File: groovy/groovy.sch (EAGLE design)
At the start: 51 parts, among them J1 USB_MICRO, J2 2_PIN_JST-XH, J3 BL, J4 PWR, J5 FLASH, P1 MICROSD, U1 MCP73831T, U2 AP7312-1833, U3 VS1053, U4 ATMEGA328PB-AUR, Y1 ABM8G-12.288MHZ-18-D2Y-T, Y2 8MHz

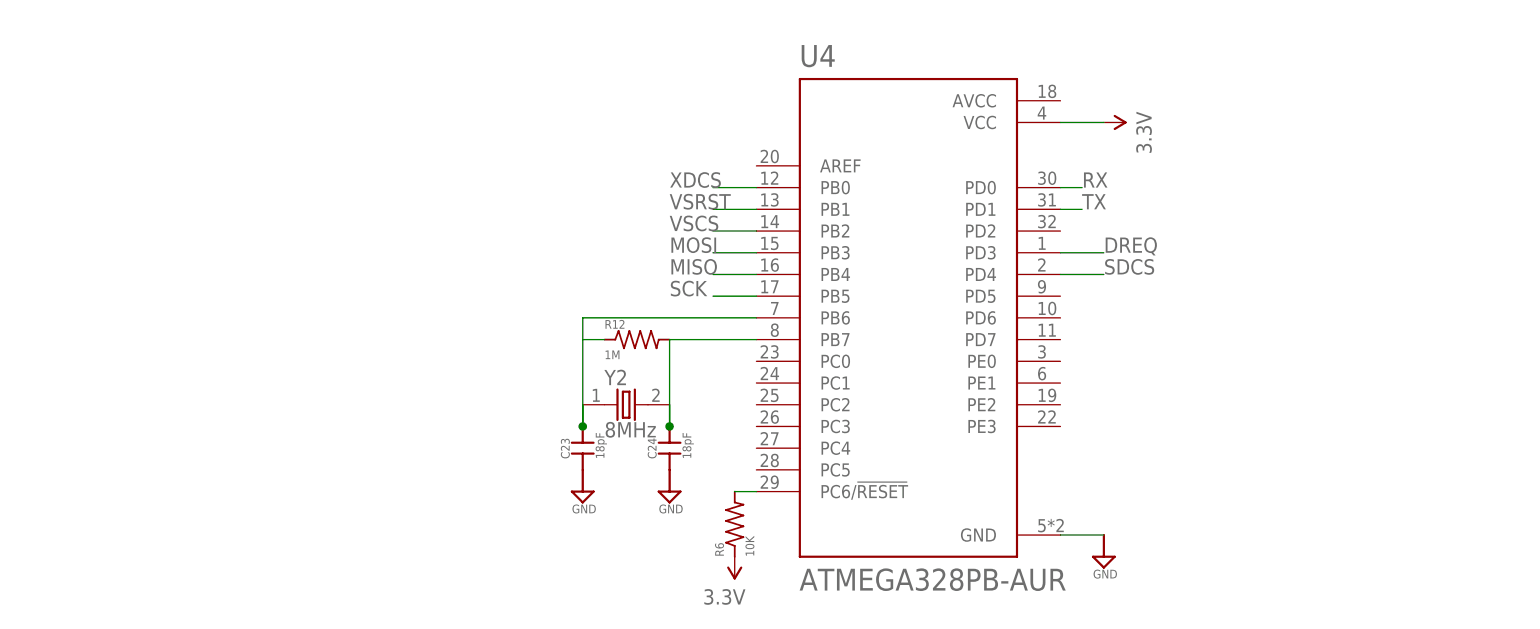
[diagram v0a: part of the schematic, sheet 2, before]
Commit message: left over commit
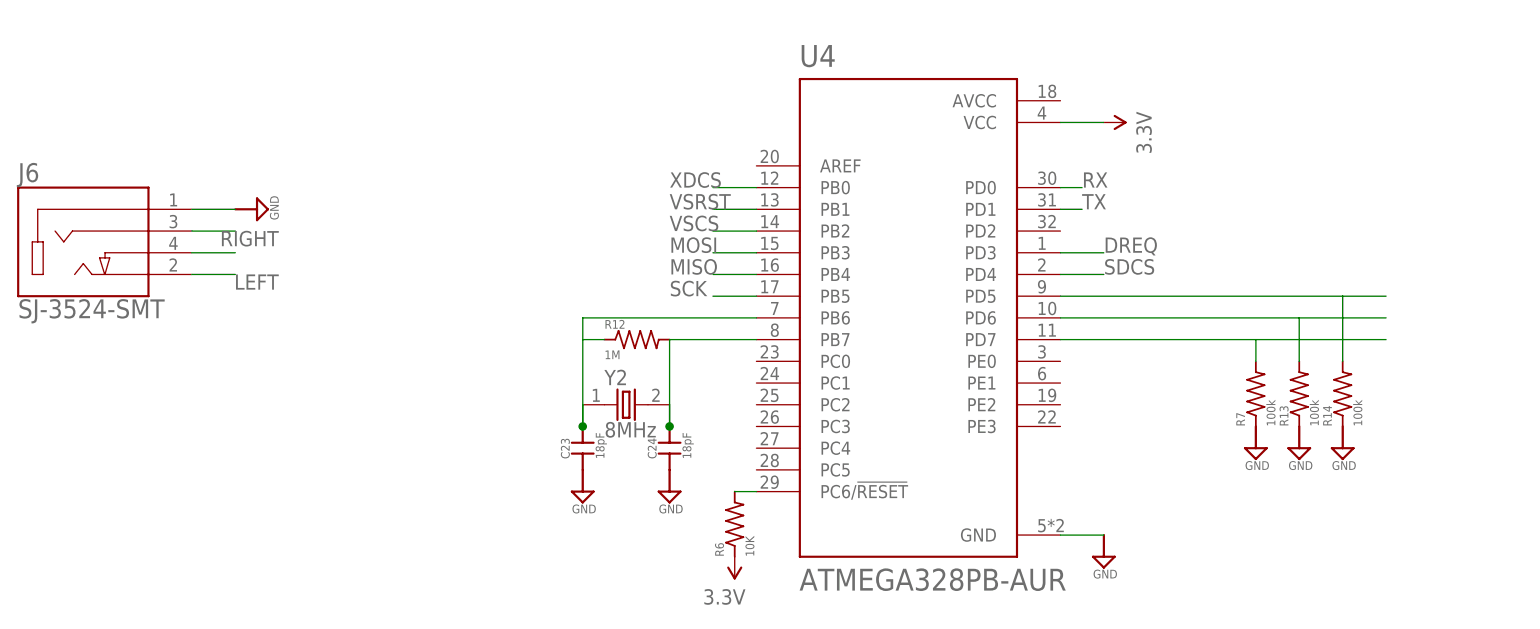
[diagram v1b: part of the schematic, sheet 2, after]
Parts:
- added J6: SJ-3524-SMT, scono:SJ-3524-SMT
- added R13, R14, R7: 100k, scono:R-US_R0603
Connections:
- new net N$10: J6.4
- new net N$11: R14.2, U4.PD5
- new net N$7: R7.2, U4.PD7
- new net N$9: R13.2, U4.PD6
- net GND: now also J6.1, R13.1, R14.1, R7.1
- net LEFT: now also J6.2
- net RIGHT: now also J6.3
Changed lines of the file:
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@@
 <part name="SUPPLY15" library="scono" deviceset="GND" device=""/>
 <part name="U$5" library="scono" deviceset="3.3V" device=""/>
+<part name="J6" library="scono" deviceset="SJ-3524-SMT" device=""/>
+<part name="SUPPLY18" library="scono" deviceset="GND" device=""/>
+<part name="R7" library="scono" deviceset="R-US_" device="R0603" value="100k"/>
+<part name="R13" library="scono" deviceset="R-US_" device="R0603" value="100k"/>
+<part name="R14" library="scono" deviceset="R-US_" device="R0603" value="100k"/>
+<part name="SUPPLY27" library="scono" deviceset="GND" device=""/>
+<part name="SUPPLY28" library="scono" deviceset="GND" device=""/>
+<part name="SUPPLY29" library="scono" deviceset="GND" device=""/>
 </parts>
 <sheets>
@@
 <instance part="SUPPLY15" gate="GND" x="200.66" y="81.28" rot="R270"/>
 <instance part="U$5" gate="G$1" x="203.2" y="71.12" rot="R90"/>
+<instance part="J6" gate="G$1" x="25.4" y="71.12"/>
+<instance part="SUPPLY18" gate="GND" x="45.72" y="76.2" rot="R90"/>
+<instance part="R7" gate="G$1" x="162.56" y="55.88" rot="R90"/>
+<instance part="R13" gate="G$1" x="167.64" y="55.88" rot="R90"/>
+<instance part="R14" gate="G$1" x="172.72" y="55.88" rot="R90"/>
+<instance part="SUPPLY27" gate="GND" x="162.56" y="48.26"/>
+<instance part="SUPPLY28" gate="GND" x="167.64" y="48.26"/>
+<instance part="SUPPLY29" gate="GND" x="172.72" y="48.26"/>
 </instances>
 <busses>
@@
 <label x="142.24" y="119.38" size="1.778" layer="95"/>
 </segment>
+<segment>
+<pinref part="J6" gate="G$1" pin="2"/>
+<wire x1="38.1" y1="68.58" x2="43.18" y2="68.58" width="0.1524" layer="91"/>
+<label x="48.26" y="68.58" size="1.778" layer="95" rot="R180"/>
+</segment>
 </net>
 <net name="GBUF" class="0">
@@
 <wire x1="142.24" y1="124.46" x2="152.4" y2="124.46" width="0.1524" layer="91"/>
 <label x="142.24" y="124.46" size="1.778" layer="95"/>
+</segment>
+<segment>
+<pinref part="J6" gate="G$1" pin="3"/>
+<wire x1="38.1" y1="73.66" x2="43.18" y2="73.66" width="0.1524" layer="91"/>
+<label x="48.26" y="73.66" size="1.778" layer="95" rot="R180"/>
 </segment>
 </net>
@@
 <pinref part="SUPPLY15" gate="GND" pin="GND"/>
 </segment>
+<segment>
+<pinref part="J6" gate="G$1" pin="1"/>
+<wire x1="38.1" y1="76.2" x2="43.18" y2="76.2" width="0.1524" layer="91"/>
+<pinref part="SUPPLY18" gate="GND" pin="GND"/>
+</segment>
+<segment>
+<pinref part="R7" gate="G$1" pin="1"/>
+<pinref part="SUPPLY27" gate="GND" pin="GND"/>
+</segment>
+<segment>
+<pinref part="R13" gate="G$1" pin="1"/>
+<pinref part="SUPPLY28" gate="GND" pin="GND"/>
+</segment>
+<segment>
+<pinref part="R14" gate="G$1" pin="1"/>
+<pinref part="SUPPLY29" gate="GND" pin="GND"/>
+</segment>
 </net>
 <net name="XTALIN" class="0">
@@
 </segment>
 </net>
+<net name="N$10" class="0">
+<segment>
+<pinref part="J6" gate="G$1" pin="4"/>
+<wire x1="38.1" y1="71.12" x2="43.18" y2="71.12" width="0.1524" layer="91"/>
+</segment>
+</net>
+<net name="N$7" class="0">
+<segment>
+<pinref part="U4" gate="G$1" pin="PD7"/>
+<wire x1="139.7" y1="60.96" x2="162.56" y2="60.96" width="0.1524" layer="91"/>
+<pinref part="R7" gate="G$1" pin="2"/>
+<wire x1="162.56" y1="60.96" x2="162.56" y2="58.42" width="0.1524" layer="91"/>
+<wire x1="162.56" y1="60.96" x2="177.8" y2="60.96" width="0.1524" layer="91"/>
+</segment>
+</net>
+<net name="N$9" class="0">
+<segment>
+<pinref part="U4" gate="G$1" pin="PD6"/>
+<wire x1="139.7" y1="63.5" x2="167.64" y2="63.5" width="0.1524" layer="91"/>
+<pinref part="R13" gate="G$1" pin="2"/>
+<wire x1="167.64" y1="63.5" x2="167.64" y2="58.42" width="0.1524" layer="91"/>
+<wire x1="167.64" y1="63.5" x2="177.8" y2="63.5" width="0.1524" layer="91"/>
+</segment>
+</net>
+<net name="N$11" class="0">
+<segment>
+<pinref part="U4" gate="G$1" pin="PD5"/>
+<wire x1="139.7" y1="66.04" x2="172.72" y2="66.04" width="0.1524" layer="91"/>
+<pinref part="R14" gate="G$1" pin="2"/>
+<wire x1="172.72" y1="66.04" x2="172.72" y2="58.42" width="0.1524" layer="91"/>
+<wire x1="172.72" y1="66.04" x2="177.8" y2="66.04" width="0.1524" layer="91"/>
+</segment>
+</net>
